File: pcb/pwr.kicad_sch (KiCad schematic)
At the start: 31 parts, among them SW6 PWR, U4 TPS63802DLAR, U5 TPS7A20xxxDQN, U6 BQ24074RGT, U7 MCP73831-2-OT

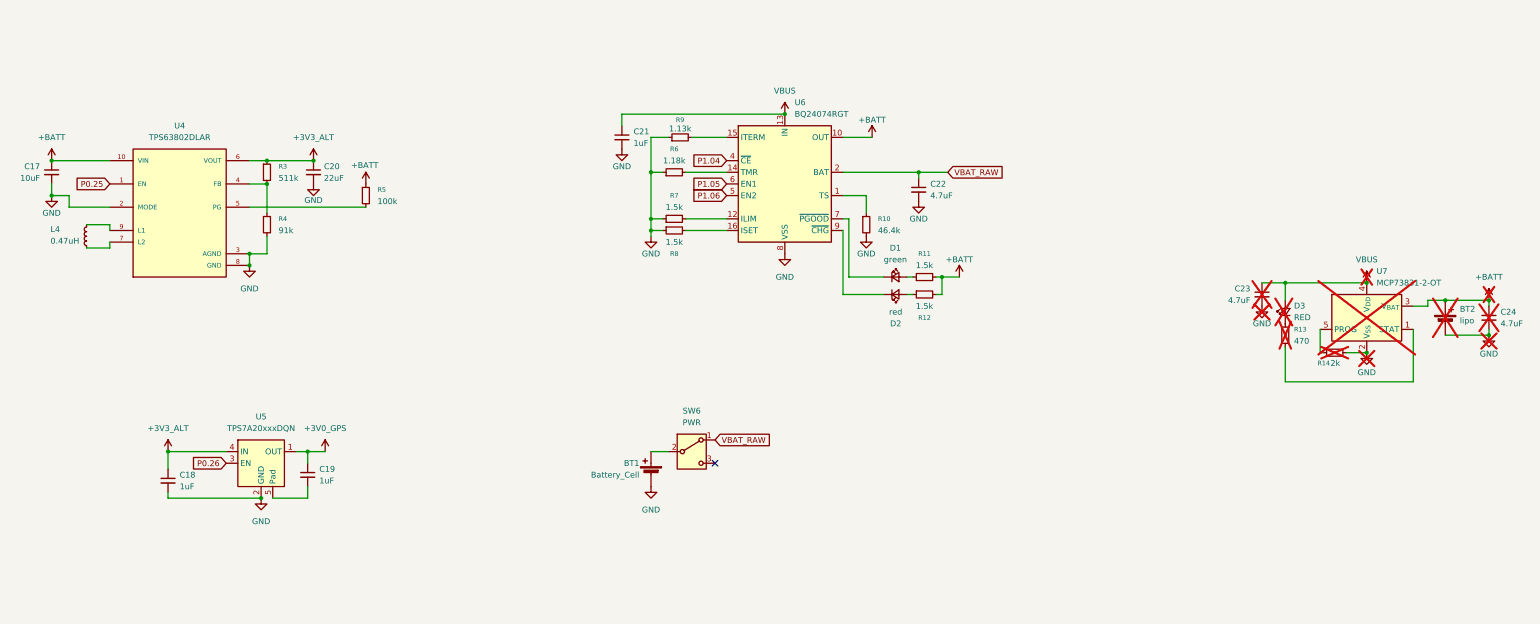
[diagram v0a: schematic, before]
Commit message: amogus
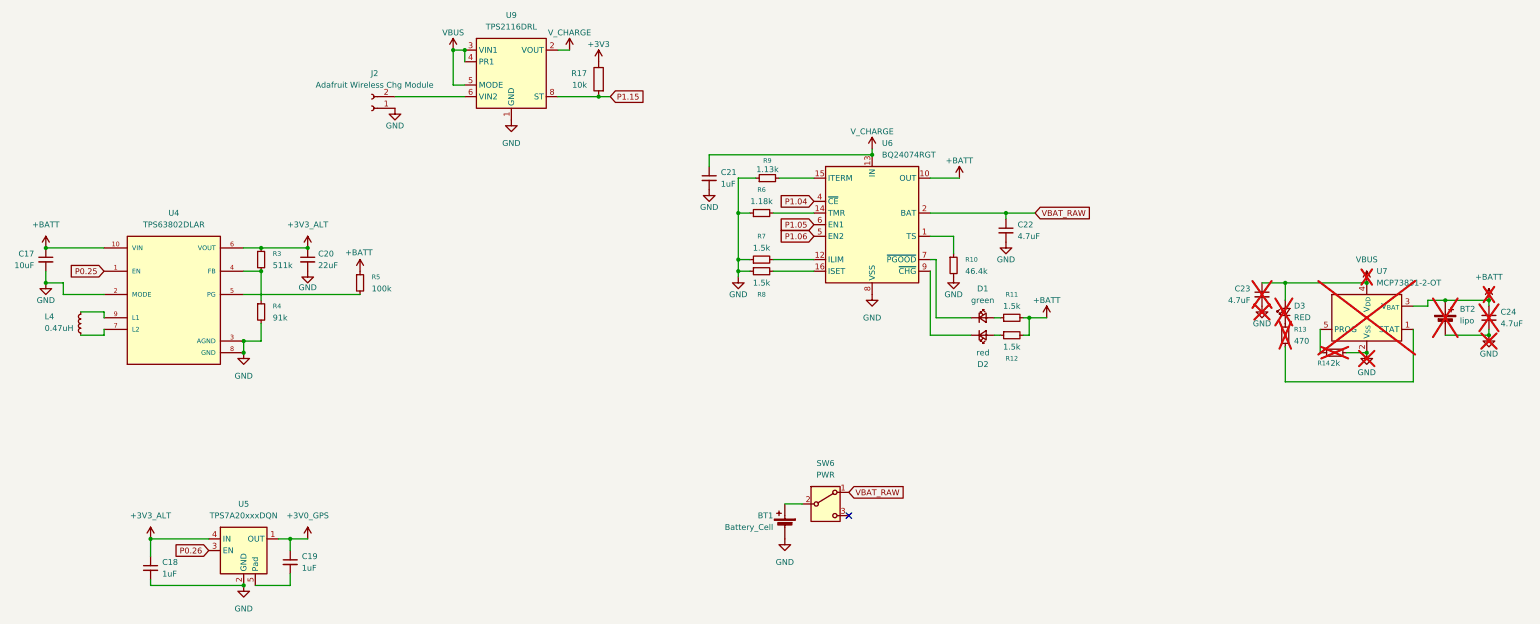
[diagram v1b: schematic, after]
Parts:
- added J2: Adafruit Wireless Chg Module, Connector_PinHeader_2.54mm:PinHeader_1x02_P2.54mm_Vertical, symbol Connector:Conn_01x02_Socket
- added R17: 10k, Resistor_SMD:R_0402_1005Metric, symbol Device:R
- added U9: TPS2116DRL, Package_TO_SOT_SMD:SOT-583-8, symbol Power_Management:TPS2116DRL
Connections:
- net GND: now also J2.1 (Pin_1), U9.1 (GND)
- net VBUS: now also U9.3 (VIN1), U9.4 (PR1), U9.5 (MODE); no longer C21.1, U6.13 (IN)
- new net: J2.2 (Pin_2), U9.6 (VIN2)
- new net +3V3: R17.1
- new net P1.15: R17.2, U9.8 (ST)
- new net V_CHARGE: C21.1, U6.13 (IN), U9.2 (VOUT), U9.7 (VOUT)
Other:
- moved on the sheet: BT1, C17, C18, C19, C20, C21, C22, D1, D2, L4, R10, R11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
